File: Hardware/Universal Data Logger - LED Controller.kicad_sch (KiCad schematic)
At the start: 0 parts

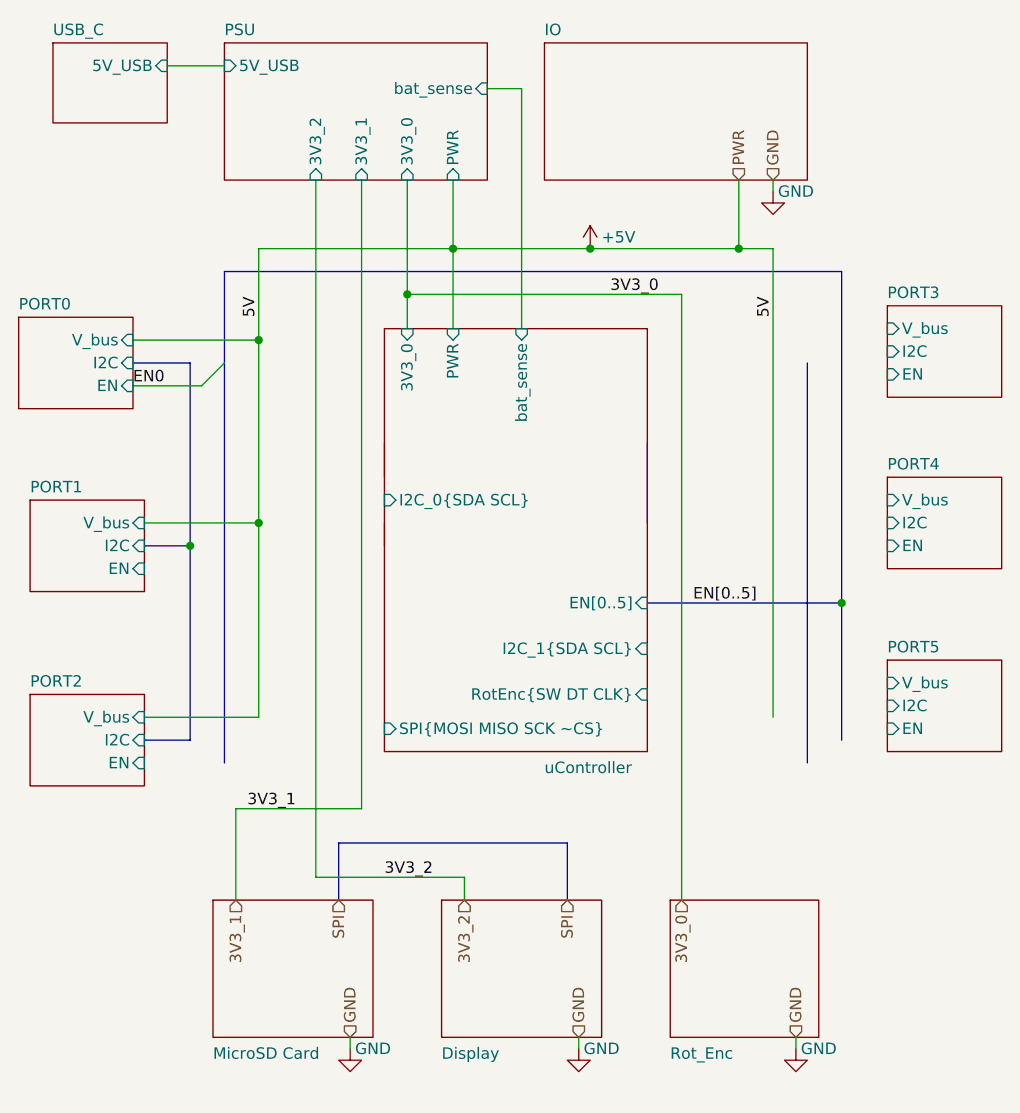
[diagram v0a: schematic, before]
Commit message: cleaned up busses
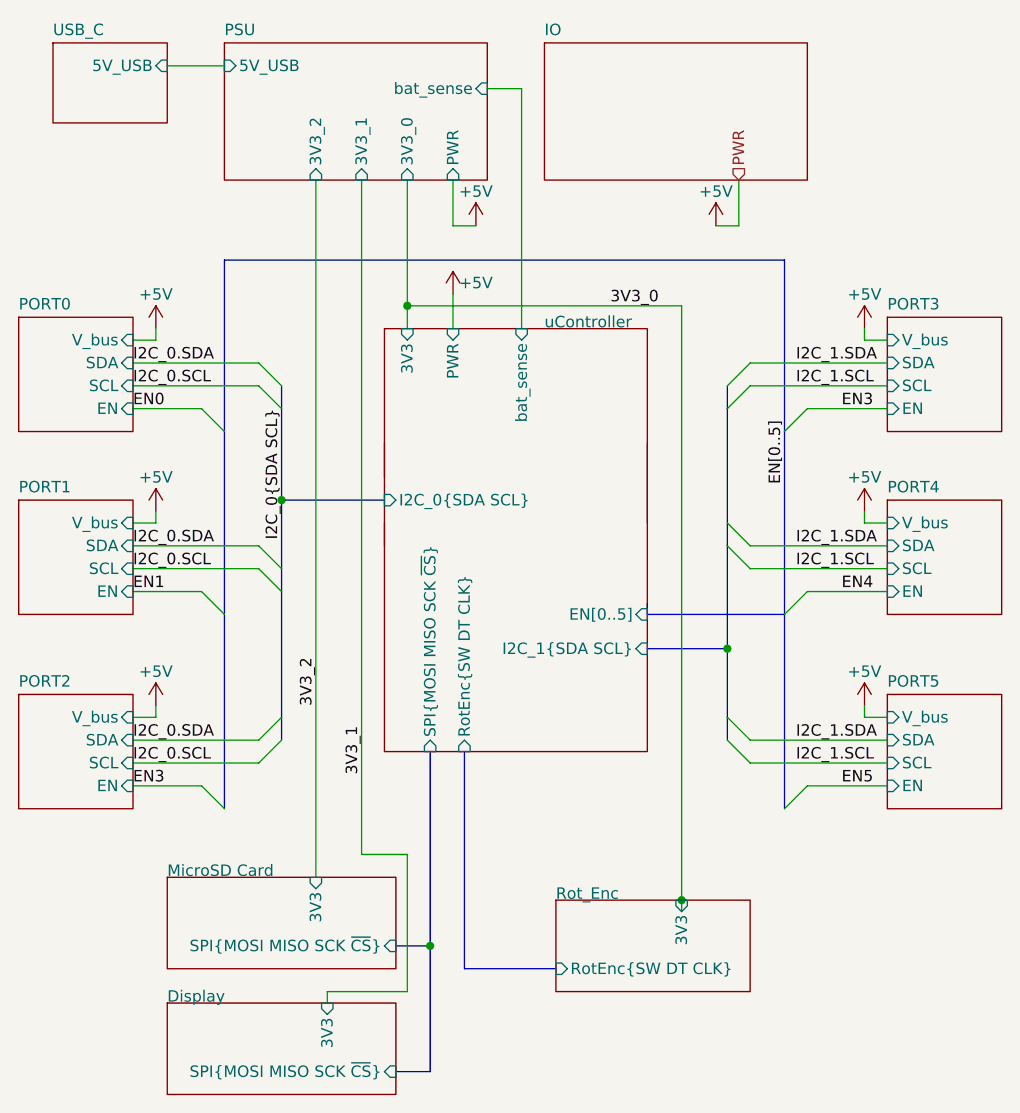
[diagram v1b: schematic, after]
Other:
- sheet Display ports: added 3V3, SPI{MOSI MISO SCK ~{CS}}; removed none
- sheet MicroSD Card ports: added 3V3, SPI{MOSI MISO SCK ~{CS}}; removed none
- sheet PORT0 ports: added SCL, SDA; removed I2C
- sheet PORT1 ports: added SCL, SDA; removed I2C
- sheet PORT2 ports: added SCL, SDA; removed I2C
- sheet PORT3 ports: added SCL, SDA; removed I2C
- sheet PORT4 ports: added SCL, SDA; removed I2C
- sheet PORT5 ports: added SCL, SDA; removed I2C
- sheet Rot_Enc ports: added 3V3, RotEnc{SW DT CLK}; removed none
- sheet uController ports: added 3V3, SPI{MOSI MISO SCK ~{CS}}; removed 3V3_0, SPI{MOSI MISO SCK ~CS}
